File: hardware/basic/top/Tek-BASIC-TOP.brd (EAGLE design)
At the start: 100 x 80 mm, 0 parts

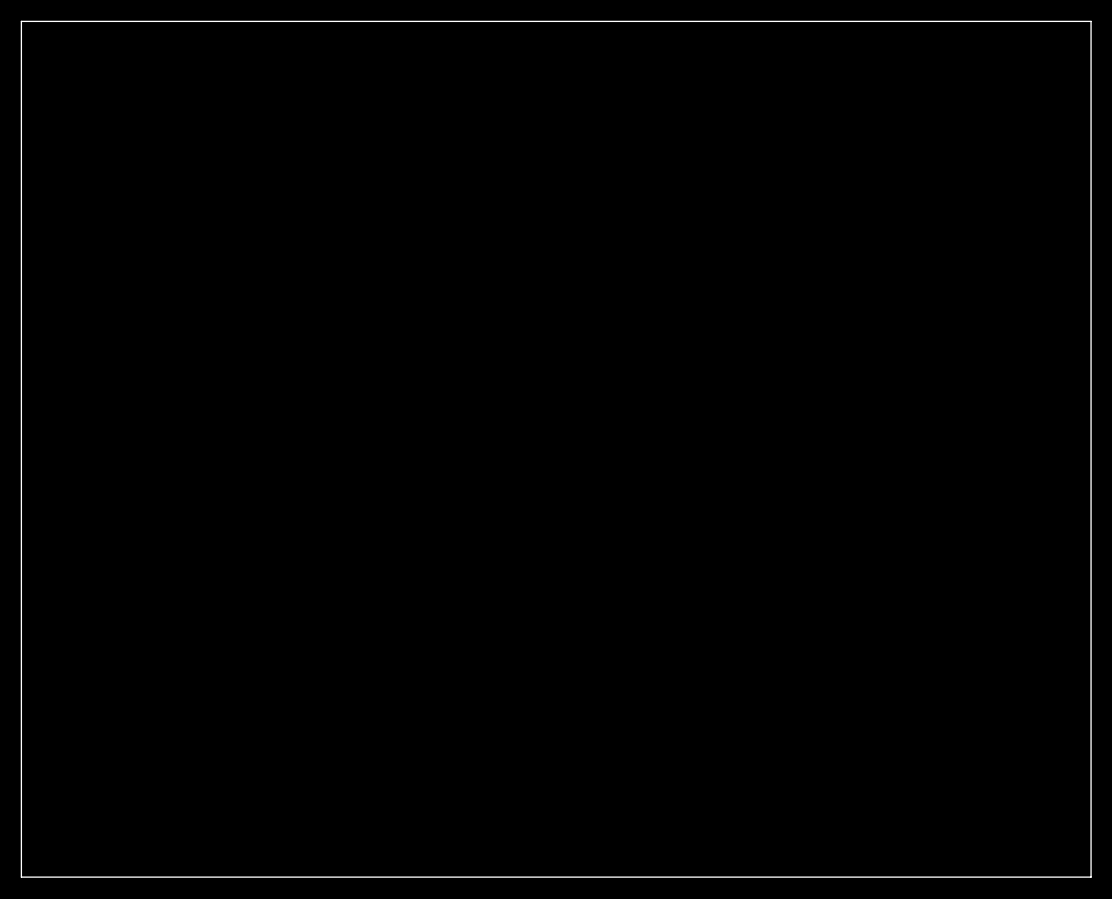
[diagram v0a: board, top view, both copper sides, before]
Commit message: Upload ot the udpdates made on the top board design: base items added on the schematic and on the board
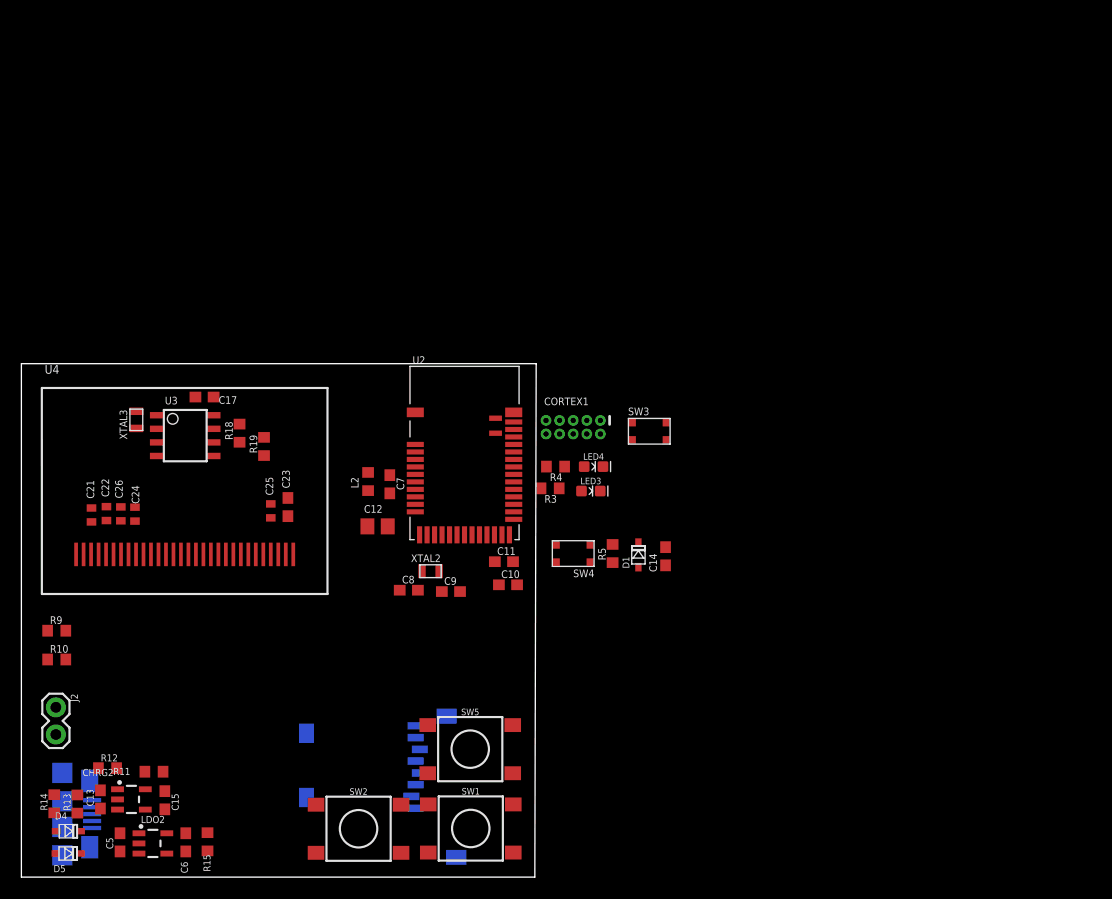
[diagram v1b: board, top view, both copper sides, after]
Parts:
- added C10, C11: 300p, LinnesLab-Passives:C0603
- added C12: 10u, LinnesLab-Passives:C0805
- added C13, C15: 4.7u, LinnesLab-Passives:C0603
- added C14: 100n, LinnesLab-Passives:C0603
- added C17, C5, C6, C7: 1u, LinnesLab-Passives:C0603
- added C21, C22, C24, C25, C26: 2.2uF, LinnesLab-Passives:C0402
- added C23: 10uF, LinnesLab-Passives:C0603
- added C8, C9: (no value), LinnesLab-Passives:C0603
- added CHRG2: MCP73831, LinnesLab-Power:SOT23-5
- added CORTEX1: CORTEX_DEBUG_PTH, LinnesLab-Connectors:2X5-PTH-1.27MM
- added D1, D4, D5: (no value), LinnesLab-DiscreteSemi:USC
- added J2: (no value), LinnesLab-Connectors:1X02
- added L2: 10u, LinnesLab-Passives:L0603
- added LDO2: MIC5504, LinnesLab-Power:SOT23-5
- added LED3: RED, LinnesLab-LED:LED-0603
- added LED4: BLUE, LinnesLab-LED:LED-0603
- added R10: 390k, LinnesLab-Passives:R0603
- added R11: (no value), LinnesLab-Passives:R0603
- added R12, R13, R14, R15: 100k, LinnesLab-Passives:R0603
- added R18, R19, R5, R9: 10k, LinnesLab-Passives:R0603
- added R3, R4: 1k, LinnesLab-Passives:R0603
- added SD2: (no value), LinnesLab-Connectors:MICROSD
- added SW1, SW2, SW5: SWITCH.MOM, LinnesLab-Switches:TACTILE_SWITCH_SMD_6.2MM_TALL
- added SW3, SW4: (no value), LinnesLab-Switches:BUTTON-GULLWING
- added U2: NRF52832_MODULE_MDBT42, LinnesLab-Microcontrollers:BLE_MODULE_RAYTAC_MDBT42
- added U3: PCF8523, LinnesLab-Clocks:SO8
- added U4: (no value), LinnesLab-Displays:UG-2864HSWEG01_0.96IN_NO-WRAPAROUND
- added USB2: USB.MICRO-BIGGERPADS, LinnesLab-Connectors:USB-MICRO-01.BIGGERPADS
- added XTAL2: 32.768kHz, LinnesLab-Clocks:2-SMD.NOLEAD.2.0MMTO1.2MM
- added XTAL3: 32.7680kHz, LinnesLab-Clocks:2-SMD.NOLEAD.2.0MMTO1.2MM
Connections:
- new net 3.3V: C12.2, C17.1, C24.2, C26.2, C6.1, CORTEX1.1, D1.-, LDO2.5, R15.2, R18.2, R19.2, R5.2, SD2.4, U2.11, U3.8, U4.6, U4.9
- new net BATT: R13.1, R14.2
- new net CD1: SD2.CD1
- new net CD2: SD2.CD2
- new net CHRG.STAT: CHRG2.1, R12.1
- new net CS.OLED: U4.13
- new net DC.OLED: U4.15
- new net DFU: SW3.3, U2.34
- new net DTR: C14.1
- new net FRST: U2.38
- new net GND: C10.2, C11.2, C12.1, C13.2, C15.1, C17.2, C23.1, C24.1, C25.1, C26.1, C5.1, C6.2, C7.2, C8.1, C9.2, CHRG2.2, CORTEX1.3, CORTEX1.5, CORTEX1.7, CORTEX1.9, J2.1, LDO2.2, LED3.C, LED4.C, R10.2, R11.1, R14.1, R15.1, R9.1, SD2.6, SD2.MT1, SD2.MT2, SW3.1, SW4.3, U2.1, U2.12, U2.24, U2.39, U3.4, U4.1, U4.10, U4.12, U4.29, U4.30, U4.8, USB2.5
- new net LED1: R3.2, U2.31
- new net LED2: R4.2, U2.33
- new net MISO: SD2.7, U2.28
- new net MOSI: SD2.3, U2.27, U4.19
- new net N$1: CHRG2.5, R11.2
- new net N$10: LED4.A, R4.1
- new net N$11: L2.1, U2.10
- new net N$12: C7.1, L2.2, U2.9
- new net N$14: CORTEX1.8
- new net N$15: R9.2, U4.11
- new net N$16: R10.1, U4.26
- new net N$17: C21.2, U4.2
- new net N$18: C21.1, U4.3
- new net N$19: C22.2, U4.4
- new net N$20: C22.1, U4.5
- new net N$21: C23.2, U4.28
- new net N$23: C25.2, U4.27
- new net N$4: C8.2, U2.13, XTAL2.P$1
- new net N$5: U3.2, XTAL3.P$1
- new net N$6: C9.1, U2.14, XTAL2.P$2
- new net N$7: U3.1, XTAL3.P$2
- new net N$9: LED3.A, R3.1
- new net P0.09/NFC1: C11.1, U2.22
- new net P0.10/NFC2: C10.1, U2.23
- new net RESET: C14.2, CORTEX1.10, D1.+, R5.1, SW4.1, U2.35
- new net RESET.OLED: U4.14
- new net RXD: U2.21
- new net SCK: SD2.5, U2.26, U4.18
- new net SCL: R18.1, U2.3, U3.6
- new net SD.CS: SD2.2
- new net SDA: R19.1, U2.2, U3.5
- new net SWCLK: CORTEX1.4, U2.36
- new net SWDIO: CORTEX1.2, U2.37
- new net SWO: CORTEX1.6, U2.32
- new net TXD: U2.19
- new net USB+: USB2.3
- new net USB-: USB2.2
- new net VBATT: U3.3
- new net VIN: C15.2, C5.2, CHRG2.4, D4.-, D5.-, LDO2.1, LDO2.3, R12.2
- new net VLIPO: C13.1, CHRG2.3, D4.+, J2.2, R13.2
- new net V_USB: D5.+, USB2.1
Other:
- board size 100 x 80 mm -> 48.1 x 48 mm
